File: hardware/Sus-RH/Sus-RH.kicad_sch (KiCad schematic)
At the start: 29 parts, among them J1 Conn_01x06, J2 Conn_01x04, J3 Conn_01x04, J4 Conn_01x04, J5 Conn_01x06, J6 Conn_01x03, J7 53307-2471

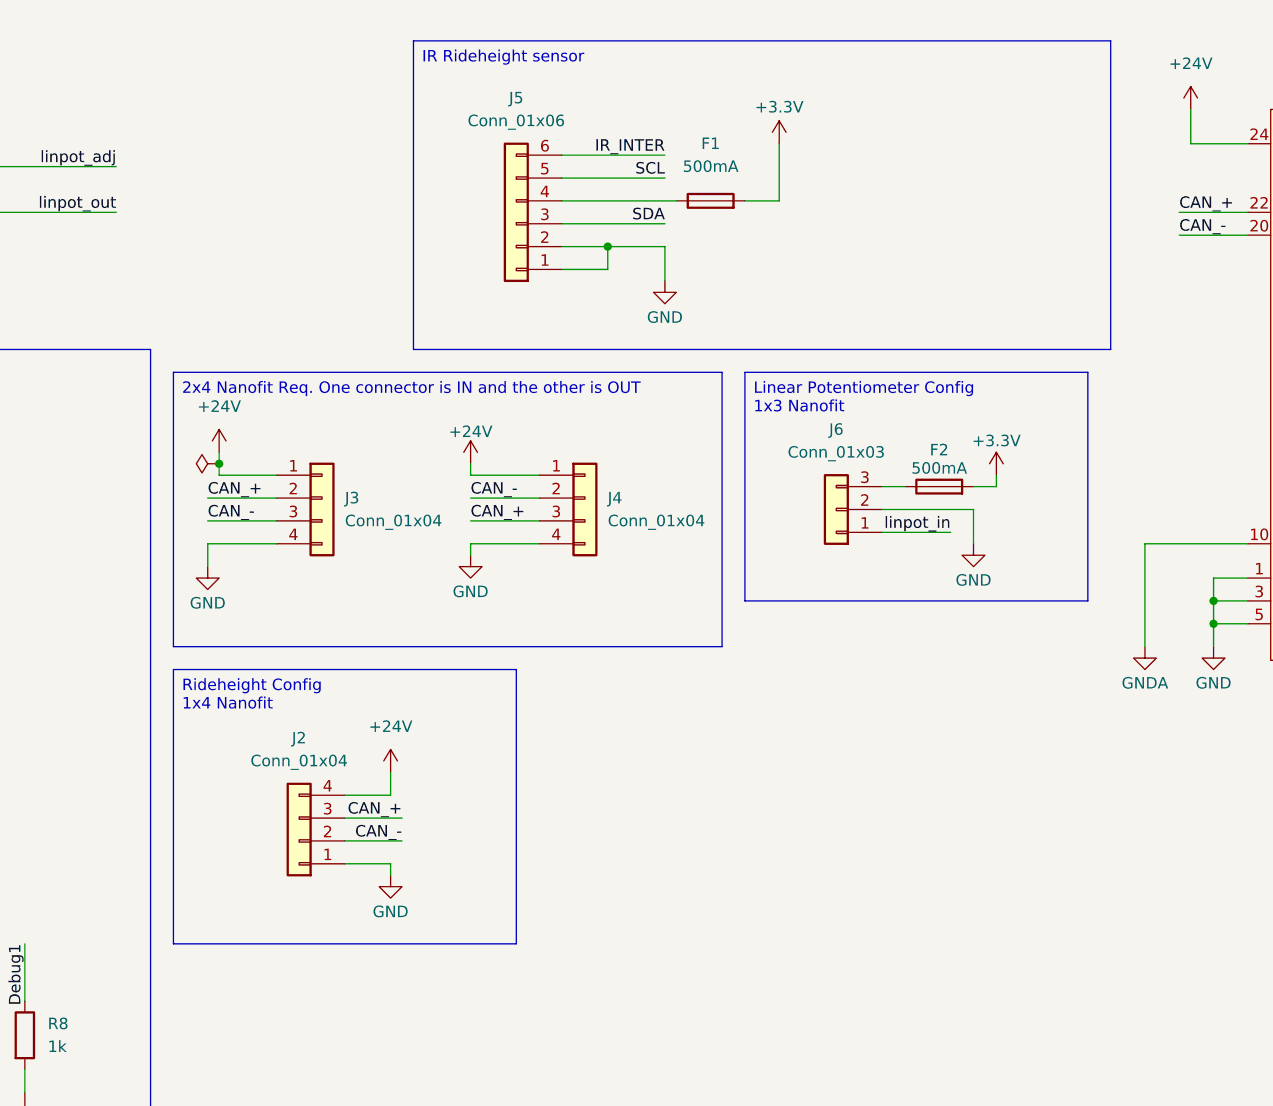
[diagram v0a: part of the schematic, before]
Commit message: made changes from review council
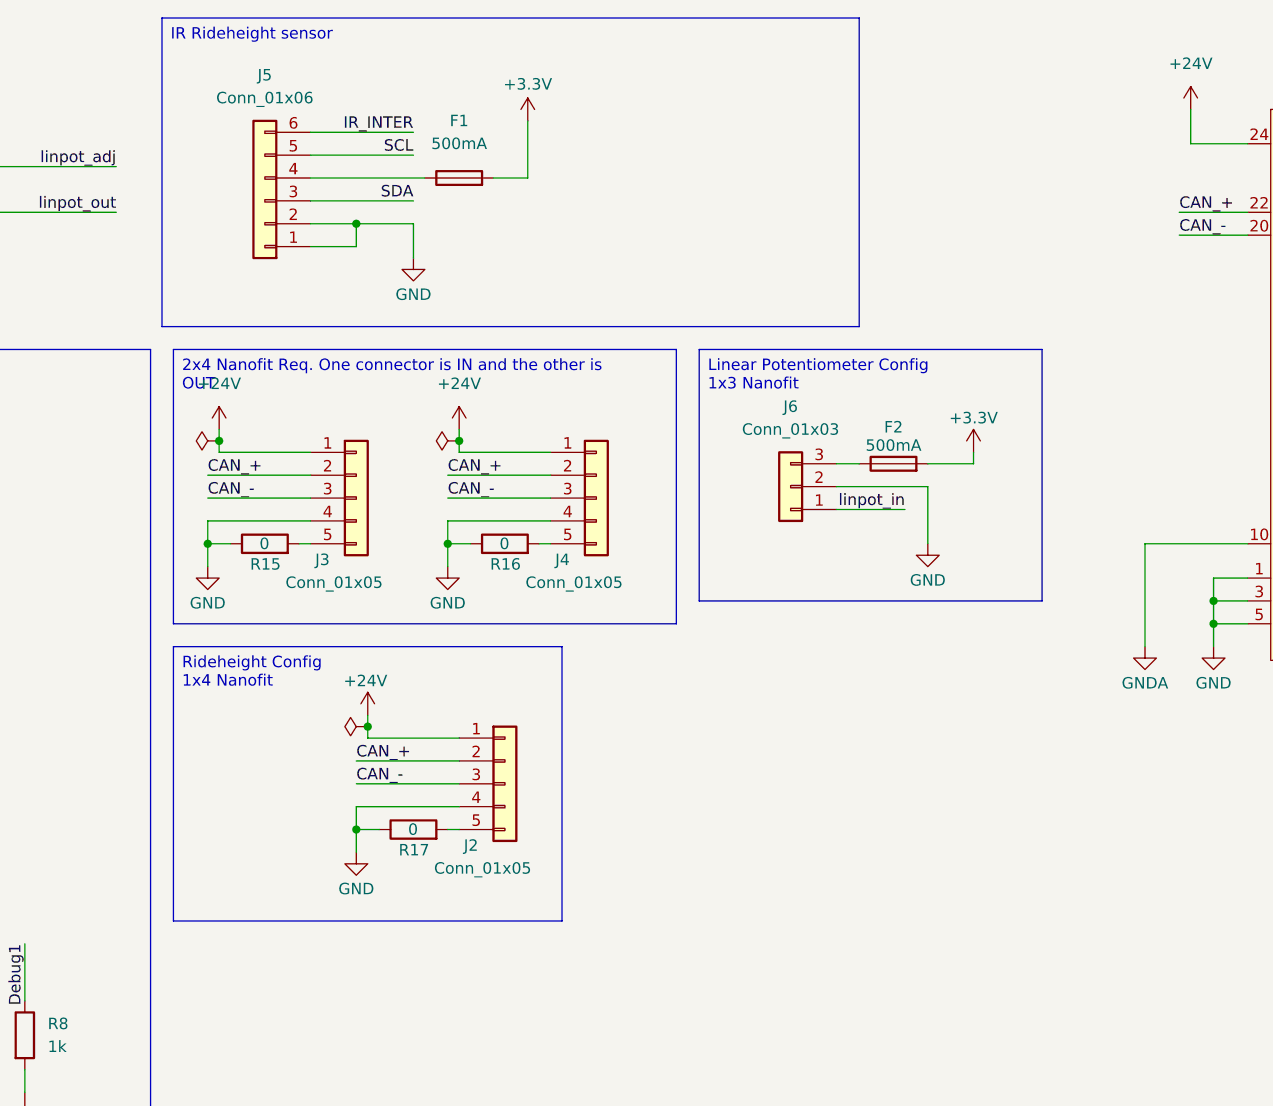
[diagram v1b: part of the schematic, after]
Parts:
- removed J2: Conn_01x04, Connector_Molex:Molex_Nano-Fit_105314-xx04_2x02_P2.50mm_Horizontal, symbol Connector_Generic:Conn_01x04
- removed J3, J4: Conn_01x04, Connector_Molex:Molex_Nano-Fit_105313-xx04_1x04_P2.50mm_Horizontal, symbol Connector_Generic:Conn_01x04
- added J2, J3, J4: Conn_01x05, Connector_Molex:Molex_Nano-Fit_105313-xx05_1x05_P2.50mm_Horizontal, symbol Connector_Generic:Conn_01x05
- added R15, R16, R17: 0, Resistor_SMD:R_0603_1608Metric_Pad0.98x0.95mm_HandSolder, symbol Device:R
- GND1: footprint TestPoint:TestPoint_Pad_1.0x1.0mm -> TestPoint:TestPoint_THTPad_2.5x2.5mm_Drill1.2mm
- GNDA1: footprint TestPoint:TestPoint_Pad_1.0x1.0mm -> TestPoint:TestPoint_THTPad_1.5x1.5mm_Drill0.7mm
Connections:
- net +24V: now also J2.1 (Pin_1), J3.1 (Pin_1), J4.1 (Pin_1)
- net CAN_+: now also J2.2 (Pin_2), J3.2 (Pin_2), J4.2 (Pin_2)
- net CAN_-: now also J2.3 (Pin_3), J3.3 (Pin_3), J4.3 (Pin_3)
- net GND: now also J2.4 (Pin_4), J3.4 (Pin_4), J4.4 (Pin_4), R15.1, R16.1, R17.1
- new net: J3.5 (Pin_5), R15.2
- new net: J2.5 (Pin_5), R17.2
- new net: J4.5 (Pin_5), R16.2
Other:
- moved on the sheet: F1, F2, J5, J6
